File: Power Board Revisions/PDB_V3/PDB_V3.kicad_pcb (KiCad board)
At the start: 2 copper layers, 208 x 137 mm, 244 parts, among them J1 1862262, J2 Conn_01x02, J3 1862262, J4 1862262, J5 1862262, Q1_1 NMOS, Q1_2 NMOS, Q1_2_1 NMOS, Q1_2_2 NMOS, Q1_2_3 NMOS, Q1_3 NMOS, Q1_4 NMOS, Q2_1 NMOS, Q2_2 NMOS, Q2_3 NMOS, Q2_4 NMOS, Q3_1 NMOS, Q3_2 NMOS, Q3_2_1 NMOS, Q3_2_2 NMOS, Q3_2_3 NMOS, Q3_2_4 NMOS, Q3_3 NMOS, Q3_4 NMOS, Q4_1 NMOS, Q4_2 NMOS, Q4_3 NMOS, Q4_4 NMOS, SW1 SW_SPST, SW10 SW_SPST, SW11 SW_SPST, SW12 SW_SPST, SW13 SW_SPST, SW14 SW_SPST, SW15 SW_SPST, SW16 SW_SPST, SW17 SW_SPST, SW18 SW_SPST, SW19 SW_SPST, SW2 SW_SPST, SW20 SW_SPST, SW21 SW_SPST, SW22 SW_SPST, SW23 SW_SPST, SW24 SW_SPST, SW25 SW_SPST, SW26 SW_SPST, SW27 SW_SPST, SW28 SW_SPST, SW29 SW_SPST, SW3 SW_SPST, SW30 SW_SPST, SW31 SW_SPST, SW32 SW_SPST, SW4 SW_SPST, SW5 SW_SPST, SW6 SW_SPST, SW7 SW_SPST, SW8 SW_SPST, SW9 SW_SPST, U1 LM5176QPWPRQ1, U2 LM5176QPWPRQ1, U3 LM5176QPWPRQ1, U4 LM5176QPWPRQ1

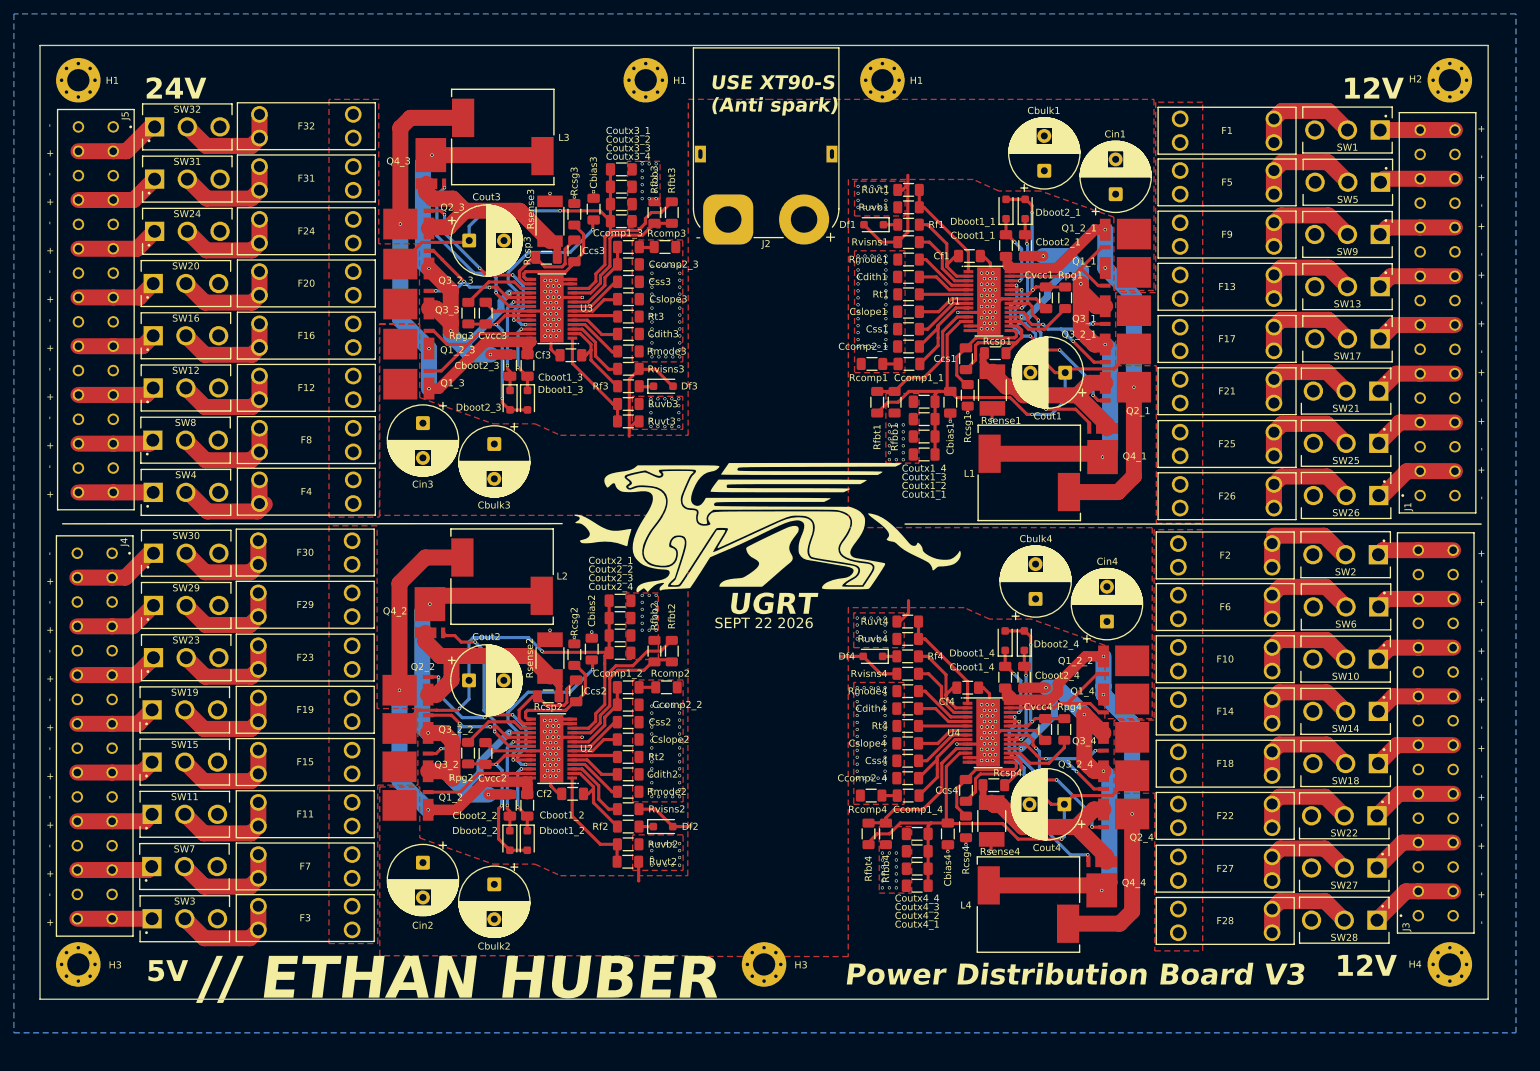
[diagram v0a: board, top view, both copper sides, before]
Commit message: Updated PDBV3
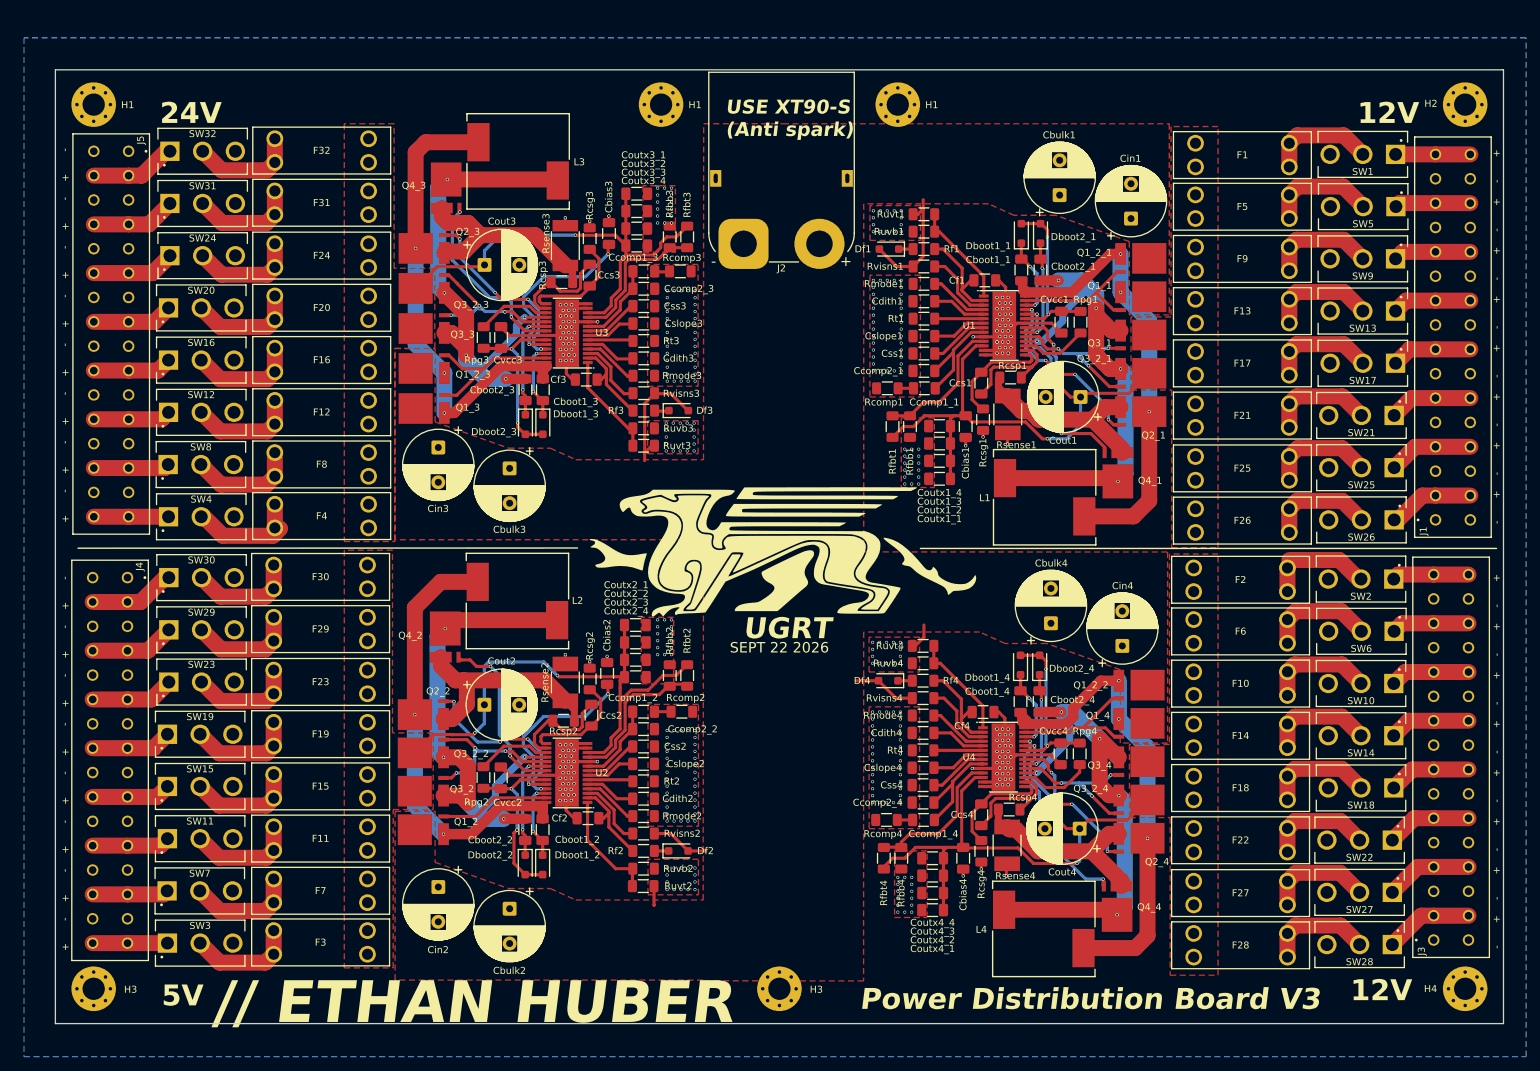
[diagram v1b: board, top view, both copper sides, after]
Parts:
- moved Cboot1_2 4.14 mm to (115.2, 130.6)
- moved Cboot2_2 4.14 mm to (112.7, 130.6)
- moved Rmode2 4.14 mm to (129.7, 128.7)
- moved Rvisns2 4.14 mm to (129.7, 131.2)
- moved Cbias1 4.14 mm to (176.0, 72.8)
- moved Cbias2 4.14 mm to (124.5, 108.2)
- moved Cbias4 4.14 mm to (175.6, 134.8)
- moved Cboot1_1 4.14 mm to (184.0, 50.2)
- moved Cboot1_4 4.14 mm to (183.8, 112.2)
- moved Cboot2_1 4.14 mm to (186.7, 50.2)
- moved Cboot2_4 4.14 mm to (186.6, 112.2)
- moved Cbulk1 4.14 mm to (189.5, 39.5)
- moved Cbulk2 4.14 mm to (110.5, 142.0)
- moved Cbulk3 4.14 mm to (110.5, 78.8)
- moved Cbulk4 4.14 mm to (188.2, 101.0)
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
